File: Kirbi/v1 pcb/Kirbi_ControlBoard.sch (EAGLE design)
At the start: 63 parts, among them U1 PCA9306_LSSOP, U2 TEENSY_3.6_DIL, U5 LM393-8-SOIC, U6 AP2114H-1.8TRG1, U7 AP2114H-3.3TRG1

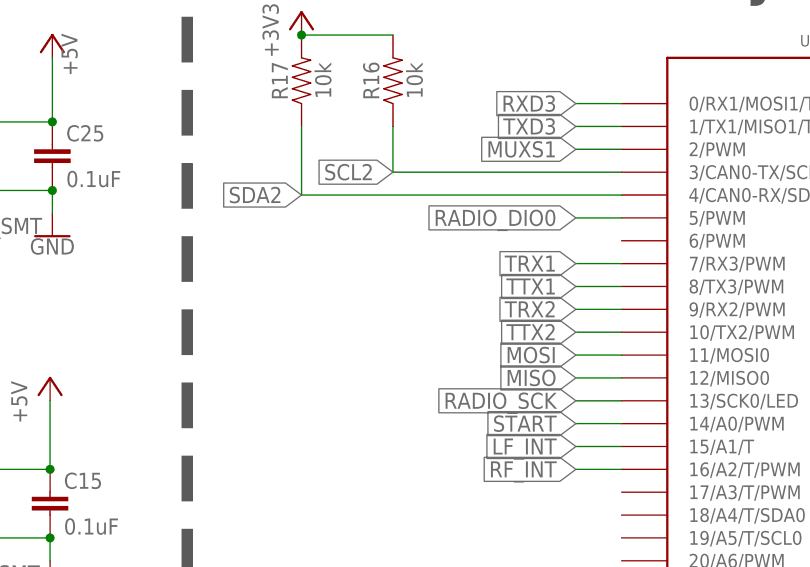
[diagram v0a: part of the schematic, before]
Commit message: Added Pull-up Resistors/Moved MUXs
Added Pull-up Resistors (1k OHM to RX line)
Added 6.2 OHM to 1.8 V LED
Moved MUXs and rerouted
Fixed SIlkscreen
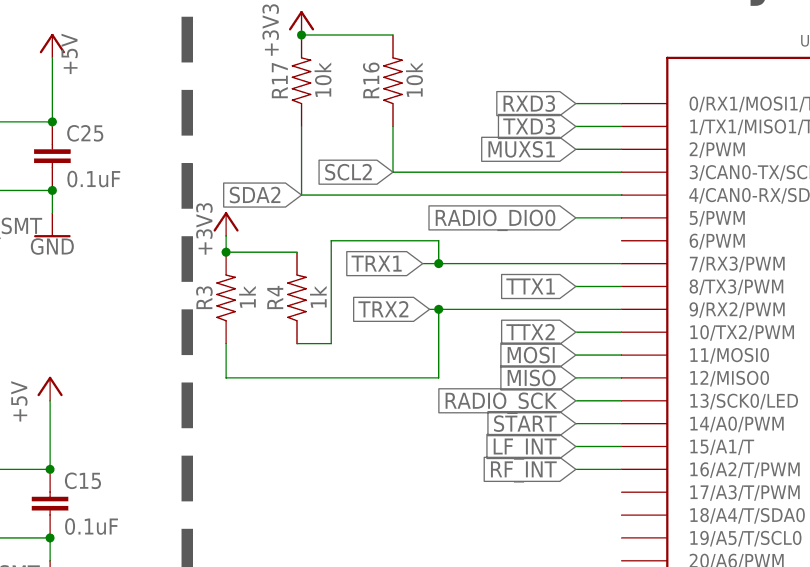
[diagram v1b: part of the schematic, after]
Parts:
- added R3, R4: 1k, SparkFun-Resistors:1KOHM-0603-1/10W-1%
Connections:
- net +3.3V: now also R3.2, R4.2
- net TRX1: now also R4.1
- net TRX2: now also R3.1
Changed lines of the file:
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@@
 <part name="F1" library="Kirbi_ControlBoard" deviceset="BEL_FUSE_C1F_3.5" device="" value="3.5"/>
 <part name="R2" library="Kirbi_ControlBoard" deviceset="6.2OHM" device="-0603-1/10W-5%" package3d_urn="urn:adsk.eagle:package:39650/1" value="6.2"/>
+<part name="R3" library="SparkFun-Resistors" library_urn="urn:adsk.eagle:library:532" deviceset="1KOHM" device="-0603-1/10W-1%" package3d_urn="urn:adsk.eagle:package:39650/1" value="1k"/>
+<part name="R4" library="SparkFun-Resistors" library_urn="urn:adsk.eagle:library:532" deviceset="1KOHM" device="-0603-1/10W-1%" package3d_urn="urn:adsk.eagle:package:39650/1" value="1k"/>
+<part name="+3V16" library="supply1" library_urn="urn:adsk.eagle:library:371" deviceset="+3V3" device=""/>
 </parts>
 <sheets>
@@
 <attribute name="VALUE" x="294.894" y="31.496" size="1.778" layer="96" font="vector" align="top-center"/>
 </instance>
+<instance part="R3" gate="G$1" x="121.158" y="214.63" smashed="yes" rot="R90">
+<attribute name="NAME" x="119.634" y="214.63" size="1.778" layer="95" font="vector" rot="R90" align="bottom-center"/>
+<attribute name="VALUE" x="122.682" y="214.63" size="1.778" layer="96" font="vector" rot="R90" align="top-center"/>
+</instance>
+<instance part="R4" gate="G$1" x="129.032" y="214.63" smashed="yes" rot="R90">
+<attribute name="NAME" x="127.508" y="214.63" size="1.778" layer="95" font="vector" rot="R90" align="bottom-center"/>
+<attribute name="VALUE" x="130.556" y="214.63" size="1.778" layer="96" font="vector" rot="R90" align="top-center"/>
+</instance>
+<instance part="+3V16" gate="G$1" x="121.158" y="224.028" smashed="yes">
+<attribute name="VALUE" x="119.634" y="219.202" size="1.778" layer="96" rot="R90"/>
+</instance>
 </instances>
 <busses>
@@
 <pinref part="C4" gate="G$1" pin="1"/>
 <junction x="236.22" y="45.72"/>
+</segment>
+<segment>
+<pinref part="+3V16" gate="G$1" pin="+3V3"/>
+<pinref part="R3" gate="G$1" pin="2"/>
+<wire x1="121.158" y1="221.488" x2="121.158" y2="219.71" width="0.1524" layer="91"/>
+<pinref part="R4" gate="G$1" pin="2"/>
+<wire x1="129.032" y1="219.71" x2="121.158" y2="219.71" width="0.1524" layer="91"/>
+<junction x="121.158" y="219.71"/>
 </segment>
 </net>
@@
 <segment>
 <pinref part="U2" gate="G$1" pin="7/RX3/PWM"/>
-<wire x1="165.1" y1="218.44" x2="160.02" y2="218.44" width="0.1524" layer="91"/>
-<label x="160.02" y="218.44" size="1.778" layer="95" rot="MR0" xref="yes"/>
+<wire x1="165.1" y1="218.44" x2="144.78" y2="218.44" width="0.1524" layer="91"/>
+<label x="143.002" y="218.44" size="1.778" layer="95" rot="MR0" xref="yes"/>
+<pinref part="R4" gate="G$1" pin="1"/>
+<wire x1="144.78" y1="218.44" x2="143.002" y2="218.44" width="0.1524" layer="91"/>
+<wire x1="129.032" y1="209.55" x2="132.842" y2="209.55" width="0.1524" layer="91"/>
+<wire x1="132.842" y1="209.55" x2="132.842" y2="220.98" width="0.1524" layer="91"/>
+<wire x1="132.842" y1="220.98" x2="144.78" y2="220.98" width="0.1524" layer="91"/>
+<wire x1="144.78" y1="220.98" x2="144.78" y2="218.44" width="0.1524" layer="91"/>
+<junction x="144.78" y="218.44"/>
 </segment>
 </net>
@@
 <segment>
 <pinref part="U2" gate="G$1" pin="9/RX2/PWM"/>
-<wire x1="165.1" y1="213.36" x2="160.02" y2="213.36" width="0.1524" layer="91"/>
-<label x="160.02" y="213.36" size="1.778" layer="95" rot="MR0" xref="yes"/>
-</segment>
-</net>
+<wire x1="165.1" y1="213.36" x2="144.78" y2="213.36" width="0.1524" layer="91"/>
+<label x="143.764" y="213.36" size="1.778" layer="95" rot="MR0" xref="yes"/>
+<pinref part="R3" gate="G$1" pin="1"/>
+<wire x1="144.78" y1="213.36" x2="143.764" y2="213.36" width="0.1524" layer="91"/>
+<wire x1="121.158" y1="209.55" x2="121.158" y2="205.74" width="0.1524" layer="91"/>
+<wire x1="121.158" y1="205.74" x2="144.78" y2="205.74" width="0.1524" layer="91"/>
+<wire x1="144.78" y1="205.74" x2="144.78" y2="213.36" width="0.1524" layer="91"/>
+<junction x="144.78" y="213.36"/>
+</segment>
+</net>
